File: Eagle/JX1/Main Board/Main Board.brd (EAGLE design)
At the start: 101.6 x 76.2 mm, 10 parts, among them U1 SN74HC595N, U2 SN74HC595N

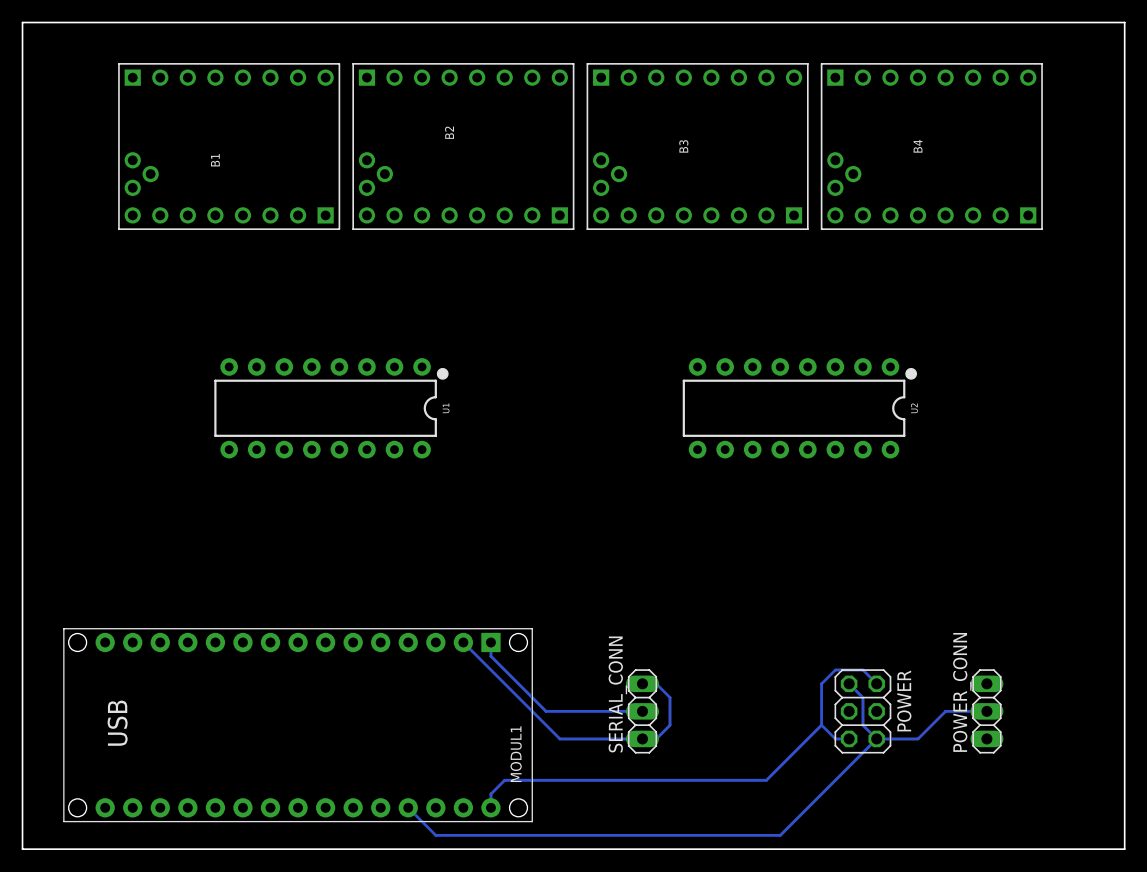
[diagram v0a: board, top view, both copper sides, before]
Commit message: Routed Main Board
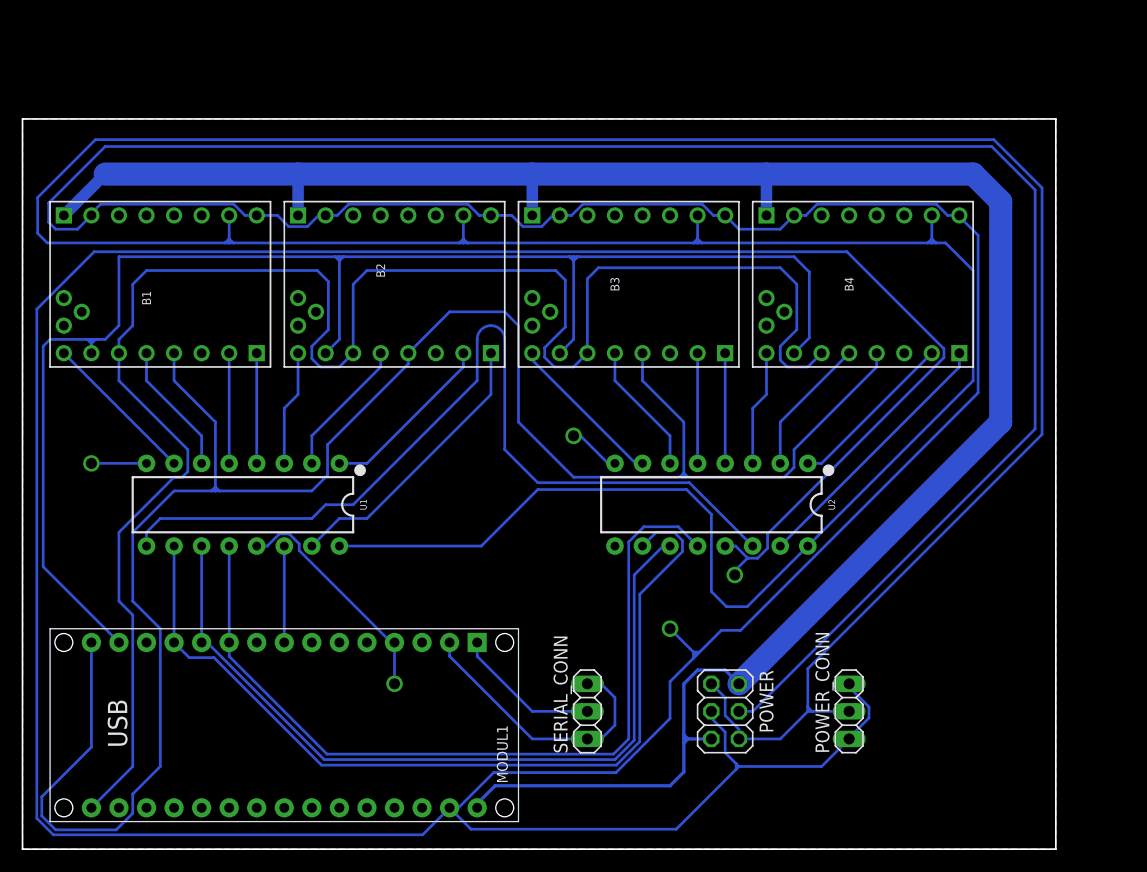
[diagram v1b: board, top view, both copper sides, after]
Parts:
- moved B1 14.2 mm to (12.7, 52.1)
- moved B2 14.2 mm to (34.3, 52.1)
- moved B3 14.2 mm to (55.9, 52.1)
- moved B4 14.2 mm to (77.5, 52.1)
- moved POWER 12.7 mm to (64.8, 12.7)
- moved POWER_CONN 12.7 mm to (76.2, 12.7)
- moved U2 11.7 mm to (63.5, 31.8)
- moved U1 11.7 mm to (20.3, 31.8)
- moved SERIAL_CONN 5.08 mm to (52.1, 12.7)
- moved MODUL1 1.27 mm to (24.1, 11.4)
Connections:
- new net NC: MODUL1.J2.4
- net +5V: no longer MODUL1.J2.4
- net N$22: now also MODUL1.J1.8; no longer MODUL1.J1.5
- net RCK: now also MODUL1.J1.10; no longer MODUL1.J1.8
- net SCL: now also MODUL1.J1.12; no longer MODUL1.J1.7
- net SSCK: now also MODUL1.J1.11; no longer MODUL1.J1.6
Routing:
- net GND: track 0.00 -> 630.0 mm, vias 0 -> 5
- net +5V: track 65.3 -> 365.1 mm
- net MISO: track 0.00 -> 182.1 mm
- net SCK: track 0.00 -> 166.9 mm
- net +12V: track 47.4 -> 193.4 mm
- net MOSI: track 0.00 -> 140.8 mm
- net SCL: track 0.00 -> 82.1 mm
- net N$2: track 0.00 -> 81.6 mm
- net RCK: track 0.00 -> 77.1 mm
- net SSCK: track 0.00 -> 73.6 mm
- net N$25: track 0.00 -> 26.1 mm
- net N$18: track 0.00 -> 24.6 mm
- net N$24: track 0.00 -> 16.4 mm
- net N$35: track 0.00 -> 15.6 mm
- net N$11: track 0.00 -> 14.7 mm
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- added copper zone on layer 1, net GND
- added copper zone on layer 16, net GND
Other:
- board size 101.6 x 76.2 mm -> 95.2 x 67.3 mm
